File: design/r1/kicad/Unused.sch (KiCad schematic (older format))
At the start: 6 parts, among them IC7 7404N, IC9 74LS01N

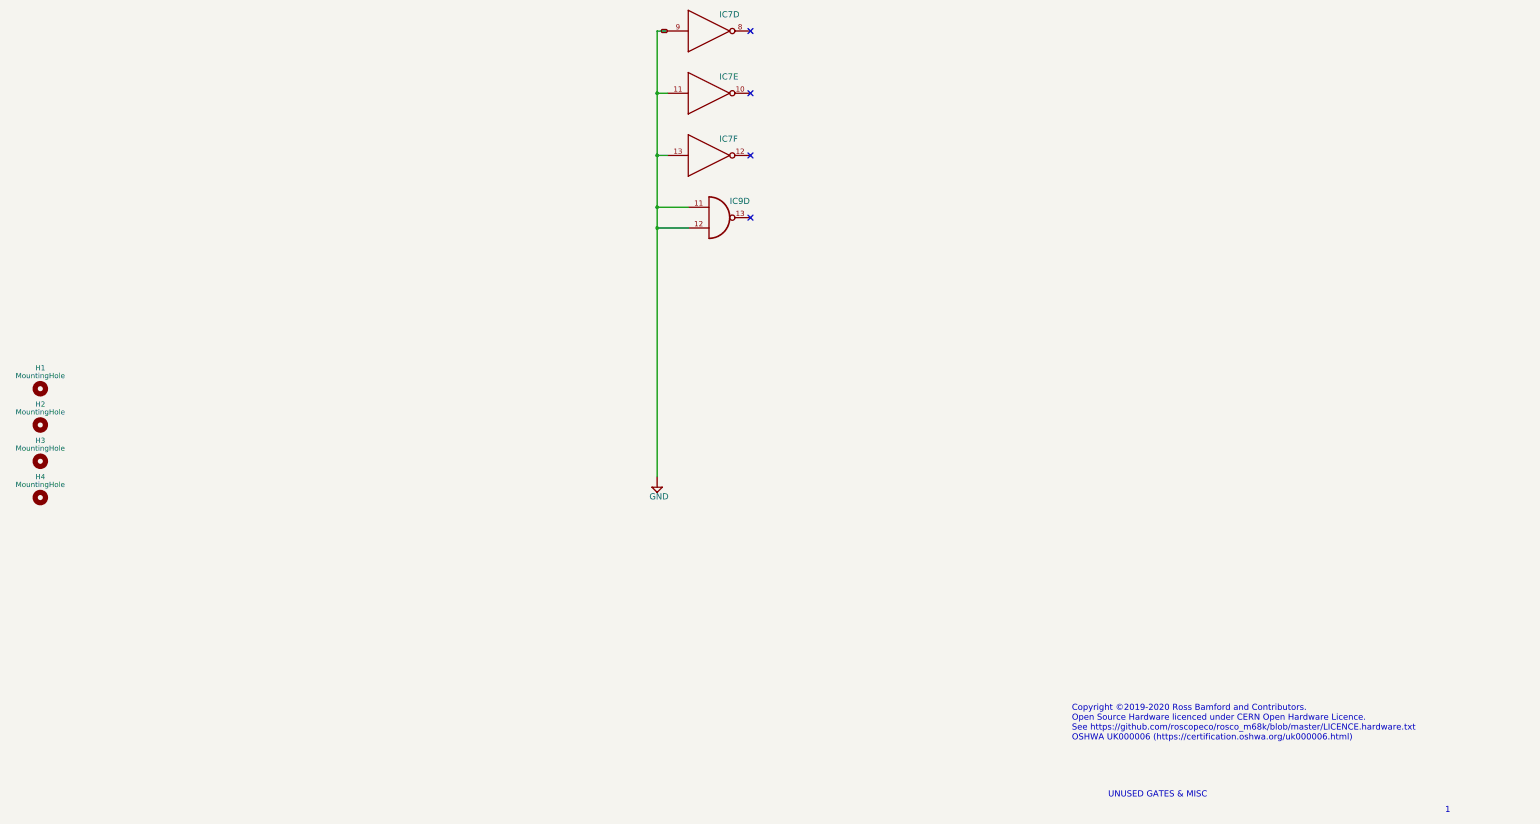
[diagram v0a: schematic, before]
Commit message: Cleanup first pass
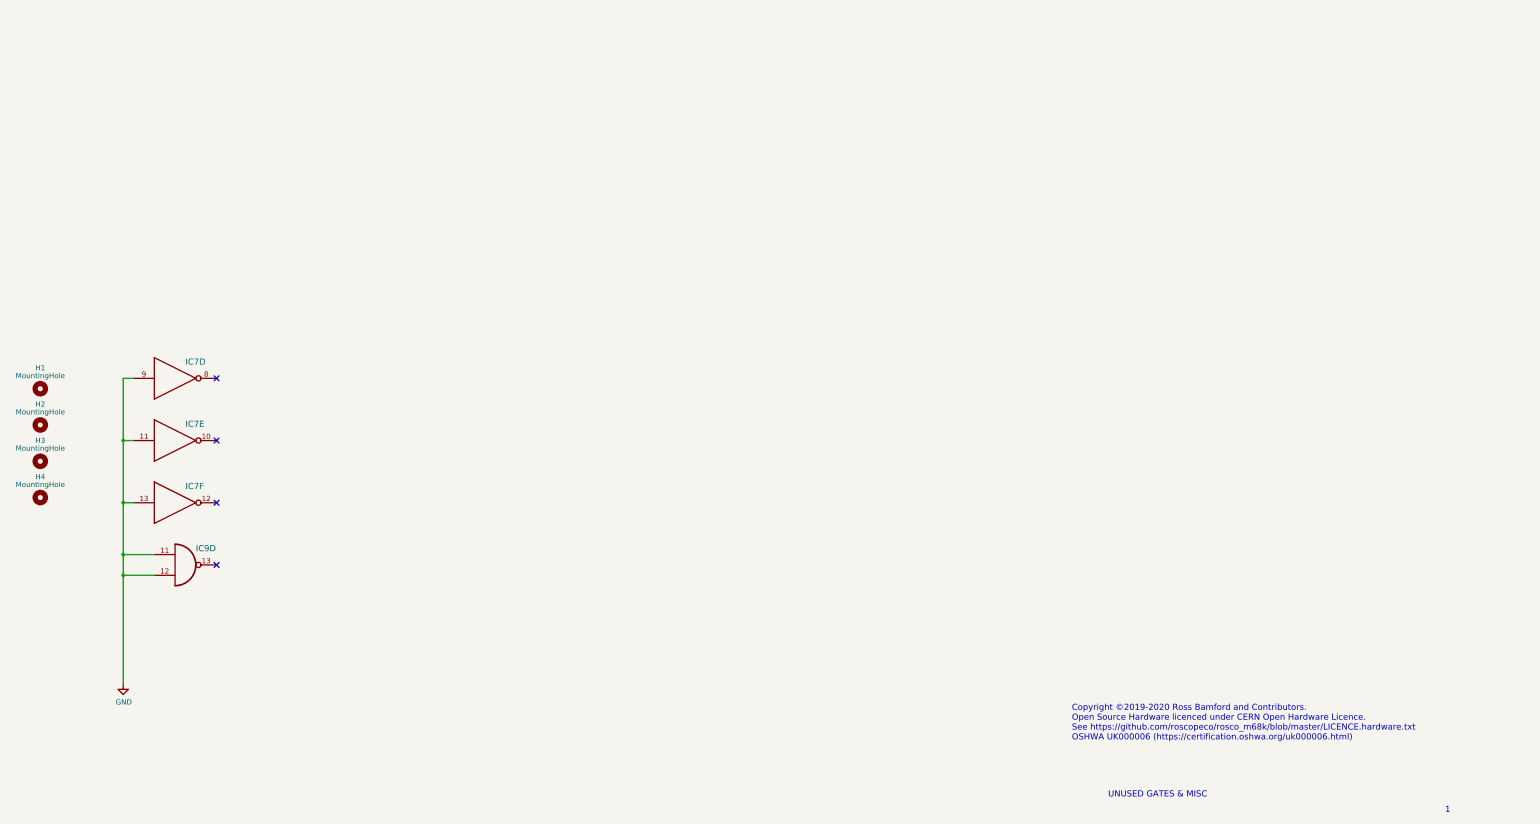
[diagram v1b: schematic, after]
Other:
- moved on the sheet: IC7D, IC7E, IC7F, IC9D
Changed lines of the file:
@@
 $EndDescr
 Wire Wire Line
-	8400 900  8300 900
+	3250 4250 3150 4250
 Wire Wire Line
-	8300 900  8300 1500
+	3150 4250 3150 4850
 Wire Wire Line
-	8300 1500 8300 2100
+	3150 4850 3150 5450
 Wire Wire Line
-	8300 2100 8300 2600
+	3150 5450 3150 5950
 Wire Wire Line
-	8300 2600 8300 2800
+	3150 5950 3150 6150
 Wire Wire Line
-	8300 2800 8300 5200
+	3450 5950 3150 5950
 Wire Wire Line
-	8600 2600 8300 2600
+	3450 6150 3150 6150
 Wire Wire Line
-	8600 2800 8300 2800
+	3250 4850 3150 4850
 Wire Wire Line
-	8400 1500 8300 1500
-Wire Wire Line
-	8400 2100 8300 2100
-Connection ~ 8300 2600
-Connection ~ 8300 2800
-Connection ~ 8300 1500
-Connection ~ 8300 2100
-Text GLabel 8400 900  0    10   BiDi ~ 0
-GND
-$Comp
-L rosco_m68k-eagle-import:GND #SUPPLY29
-U 1 1 0331A01D
-P 8300 5300
-AR Path="/0331A01D" Ref="#SUPPLY29"  Part="1"
-AR Path="/5E53BCCF/0331A01D" Ref="#SUPPLY029"  Part="1"
-F 0 "#SUPPLY029" H 8300 5300 50  0001 C CNN
-F 1 "GND" H 8225 5175 59  0000 L BNN
-F 2 "" H 8300 5300 50  0001 C CNN
-F 3 "" H 8300 5300 50  0001 C CNN
-	1    8300 5300
-	1    0    0    -1
-$EndComp
+	3250 5450 3150 5450
+Connection ~ 3150 5950
+Connection ~ 3150 6150
+Connection ~ 3150 4850
+Connection ~ 3150 5450
 $Comp
 L rosco_m68k-eagle-import:7401N IC9
 U 4 1 F64B6C48
-P 8900 2700
+P 3750 6050
 AR Path="/F64B6C48" Ref="IC9"  Part="4"
 AR Path="/5E53BCCF/F64B6C48" Ref="IC9"  Part="4"
-F 0 "IC9" H 9000 2825 59  0000 L BNN
-F 1 "74LS01N" H 9000 2500 59  0001 L BNN
-F 2 "rosco_m68k:DIL14" H 8900 2700 50  0001 C CNN
-F 3 "" H 8900 2700 50  0001 C CNN
-	4    8900 2700
+F 0 "IC9" H 3850 6175 59  0000 L BNN
+F 1 "74LS01N" H 3850 5850 59  0001 L BNN
+F 2 "rosco_m68k:DIL14" H 3750 6050 50  0001 C CNN
+F 3 "" H 3750 6050 50  0001 C CNN
+	4    3750 6050
 	1    0    0    -1
 $EndComp
@@
 L rosco_m68k-eagle-import:7404N IC7
 U 4 1 46D5F877
-P 8800 900
+P 3650 4250
 AR Path="/46D5F877" Ref="IC7"  Part="4"
 AR Path="/5E53BCCF/46D5F877" Ref="IC7"  Part="4"
-F 0 "IC7" H 8900 1025 59  0000 L BNN
-F 1 "7404N" H 8900 700 59  0001 L BNN
-F 2 "rosco_m68k:DIL14" H 8800 900 50  0001 C CNN
-F 3 "" H 8800 900 50  0001 C CNN
-	4    8800 900
+F 0 "IC7" H 3750 4375 59  0000 L BNN
+F 1 "7404N" H 3750 4050 59  0001 L BNN
+F 2 "rosco_m68k:DIL14" H 3650 4250 50  0001 C CNN
+F 3 "" H 3650 4250 50  0001 C CNN
+	4    3650 4250
 	1    0    0    -1
 $EndComp
@@
 L rosco_m68k-eagle-import:7404N IC7
 U 5 1 46D5F873
-P 8800 1500
+P 3650 4850
 AR Path="/46D5F873" Ref="IC7"  Part="5"
 AR Path="/5E53BCCF/46D5F873" Ref="IC7"  Part="5"
-F 0 "IC7" H 8900 1625 59  0000 L BNN
-F 1 "7404N" H 8900 1300 59  0001 L BNN
-F 2 "rosco_m68k:DIL14" H 8800 1500 50  0001 C CNN
-F 3 "" H 8800 1500 50  0001 C CNN
-	5    8800 1500
+F 0 "IC7" H 3750 4975 59  0000 L BNN
+F 1 "7404N" H 3750 4650 59  0001 L BNN
+F 2 "rosco_m68k:DIL14" H 3650 4850 50  0001 C CNN
+F 3 "" H 3650 4850 50  0001 C CNN
+	5    3650 4850
 	1    0    0    -1
 $EndComp
@@
 L rosco_m68k-eagle-import:7404N IC7
 U 6 1 46D5F87F
-P 8800 2100
+P 3650 5450
 AR Path="/46D5F87F" Ref="IC7"  Part="6"
 AR Path="/5E53BCCF/46D5F87F" Ref="IC7"  Part="6"
-F 0 "IC7" H 8900 2225 59  0000 L BNN
-F 1 "7404N" H 8900 1900 59  0001 L BNN
-F 2 "rosco_m68k:DIL14" H 8800 2100 50  0001 C CNN
-F 3 "" H 8800 2100 50  0001 C CNN
-	6    8800 2100
+F 0 "IC7" H 3750 5575 59  0000 L BNN
+F 1 "7404N" H 3750 5250 59  0001 L BNN
+F 2 "rosco_m68k:DIL14" H 3650 5450 50  0001 C CNN
+F 3 "" H 3650 5450 50  0001 C CNN
+	6    3650 5450
 	1    0    0    -1
 $EndComp
-NoConn ~ 9200 900
-NoConn ~ 9200 1500
-NoConn ~ 9200 2100
-NoConn ~ 9200 2700
+NoConn ~ 4050 4250
+NoConn ~ 4050 4850
+NoConn ~ 4050 5450
+NoConn ~ 4050 6050
 $Comp
 L Mechanical:MountingHole H1
@@
 Text Notes 15900 8450 0    59   ~ 0
 1
+$Comp
+L power:GND #PWR?
+U 1 1 5FD5F919
+P 3150 7200
+F 0 "#PWR?" H 3150 6950 50  0001 C CNN
+F 1 "GND" H 3155 7027 50  0000 C CNN
+F 2 "" H 3150 7200 50  0001 C CNN
+F 3 "" H 3150 7200 50  0001 C CNN
+	1    3150 7200
+	1    0    0    -1
+$EndComp
+Wire Wire Line
+	3150 6150 3150 7200
 $EndSCHEMATC
